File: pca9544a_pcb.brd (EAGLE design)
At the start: 45 x 45 mm, 3 parts, among them IC1 PCA9544ABS

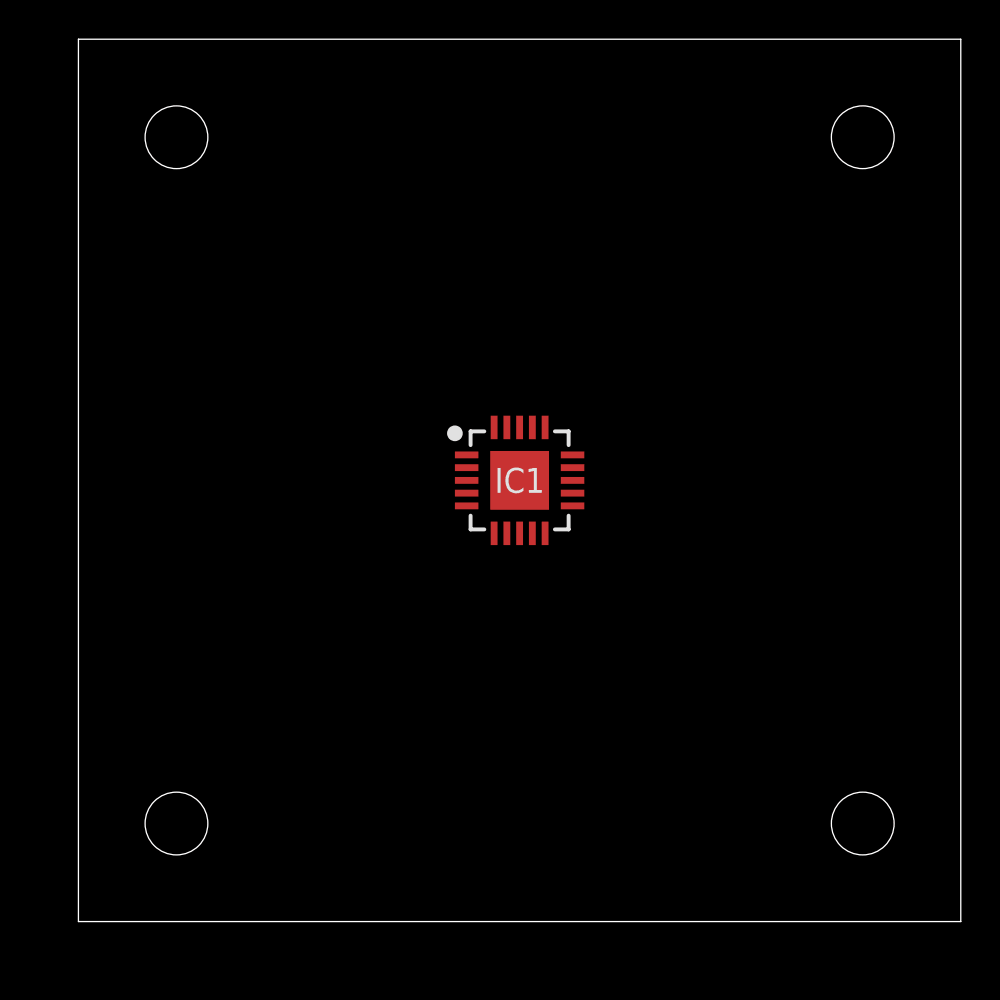
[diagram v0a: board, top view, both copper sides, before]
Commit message: add submodules
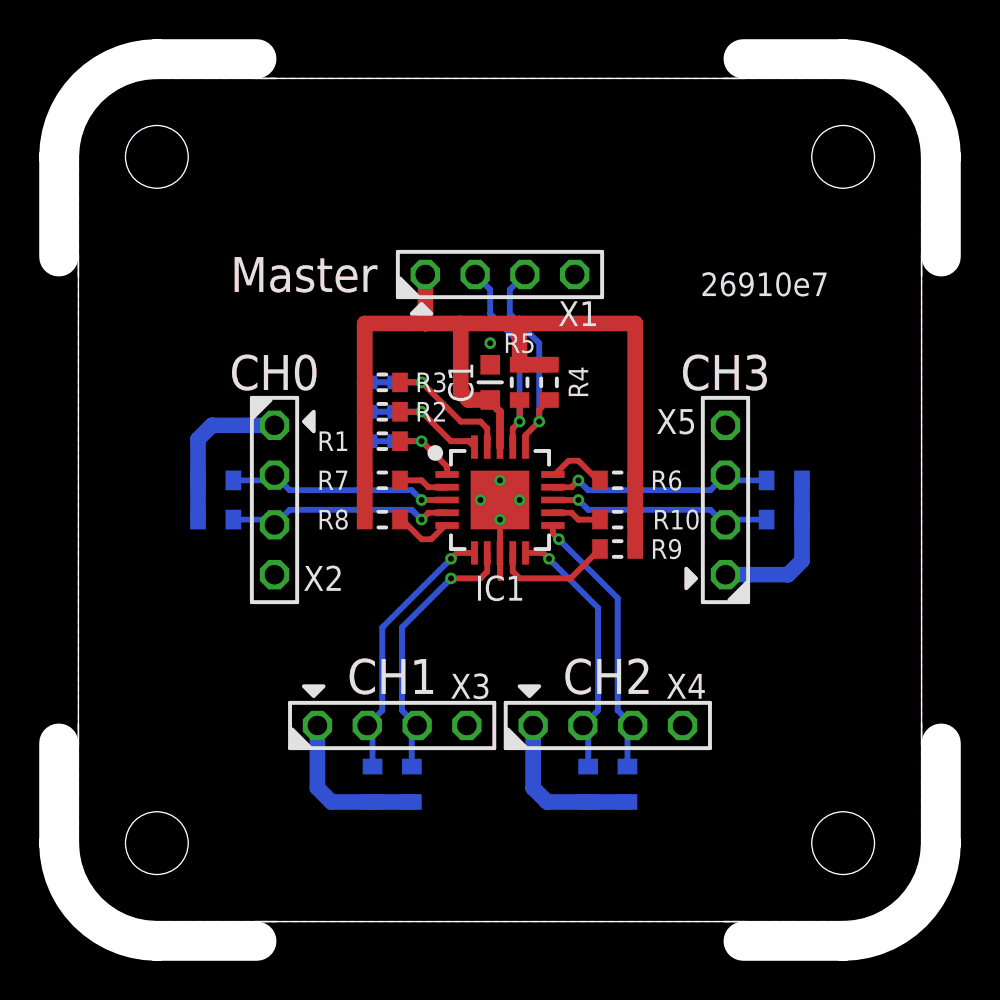
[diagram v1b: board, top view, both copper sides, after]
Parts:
- removed B1: UNIVERSALBOARD-45, mylib:BOARD-AKI-45
- added C1: (no value), mylib:CR-1608
- added P1, P2, P3, P4: (no value), mylib:PCB-CORNER
- added R1, R10, R11, R12, R13, R14, R15, R16, R17, R18, R2, R3, R4, R5, R6, R7, R8, R9: (no value), mylib:R-1608-PADPAD
- added R19, R20, R21: (no value), mylib:R0402SHORT
- added X1, X2, X3, X4, X5: TSW-104-02-S-S, con-samtec.local:TSW-104-02-S-S
- GIT1: value (none) -> 26910e7; device git-revision:GIT-REVISION_1.7 -> git-revision:GIT-REVISION_1.2
- moved GIT1 28.2 mm to (35.0, 32.5)
- moved IC1 1.41 mm to (21.5, 21.5)
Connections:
- new net GND: C1.2, IC1.8, IC1.EP, R19.1, R19.2, R20.1, R20.2, R21.1, R21.2, X1.4, X2.4, X3.4, X4.4, X5.4
- new net N$1: IC1.1, R1.1, R19.3
- new net N$10: IC1.7, R14.1, X3.3
- new net N$11: IC1.6, R13.1, X3.2
- new net N$12: IC1.5, R8.1
- new net N$13: IC1.11, R16.1, X4.3
- new net N$14: IC1.10, R15.1, X4.2
- new net N$15: IC1.9, R9.1
- new net N$16: IC1.14, R18.1, X5.3
- new net N$17: IC1.13, R17.1, X5.2
- new net N$18: IC1.12, R10.1
- new net N$19: R11.2, R12.2, X2.1
- new net N$2: IC1.20, R2.1, R20.3
- new net N$20: R13.2, R14.2, X3.1
- new net N$21: R15.2, R16.2, X4.1
- new net N$22: R17.2, R18.2, X5.1
- new net N$3: IC1.19, R21.3, R3.1
- new net N$4: IC1.16, R4.1, X1.3
- new net N$5: IC1.17, R5.1, X1.2
- new net N$6: IC1.15, R6.1
- new net N$7: IC1.4, R12.1, X2.3
- new net N$8: IC1.3, R11.1, X2.2
- new net N$9: IC1.2, R7.1
- new net VCC: C1.1, IC1.18, R1.2, R10.2, R2.2, R3.2, R4.2, R5.2, R6.2, R7.2, R8.2, R9.2, X1.1
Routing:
- net VCC: track 0.00 -> 49.4 mm
- net N$13: track 0.00 -> 14.1 mm, vias 0 -> 1
- net N$10: track 0.00 -> 14.0 mm, vias 0 -> 1
- net N$11: track 0.00 -> 13.8 mm, vias 0 -> 1
- net N$14: track 0.00 -> 13.4 mm, vias 0 -> 1
- net N$7: track 0.00 -> 11.7 mm, vias 0 -> 1
- net N$16: track 0.00 -> 11.7 mm, vias 0 -> 1
- net N$8: track 0.00 -> 11.5 mm, vias 0 -> 1
- net N$17: track 0.00 -> 11.5 mm, vias 0 -> 1
- net N$4: track 0.00 -> 11.3 mm, vias 0 -> 1
- net N$5: track 0.00 -> 11.0 mm, vias 0 -> 1
- net N$21: track 0.00 -> 8.29 mm
- net N$20: track 0.00 -> 8.29 mm
- net N$19: track 0.00 -> 8.29 mm
- net N$22: track 0.00 -> 8.29 mm
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- added copper zone on layer 1, net GND
- added copper zone on layer 16, net GND
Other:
- board size 45 x 45 mm -> 43 x 43 mm
- board text added: "@_K4ZUKI_"
- board text added: "CH0"
- board text added: "CH1"
- board text added: "CH2"
- board text added: "CH3"
- board text added: "Master"
- board text added: "PCA9544A Breakout"
